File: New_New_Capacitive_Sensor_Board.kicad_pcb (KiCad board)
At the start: 4 copper layers, 23.9 x 21 mm, 17 parts, among them J1 Conn_01x04_Pin, J2 Conn_01x04_Pin, U1 FDC2212QDNTTQ1

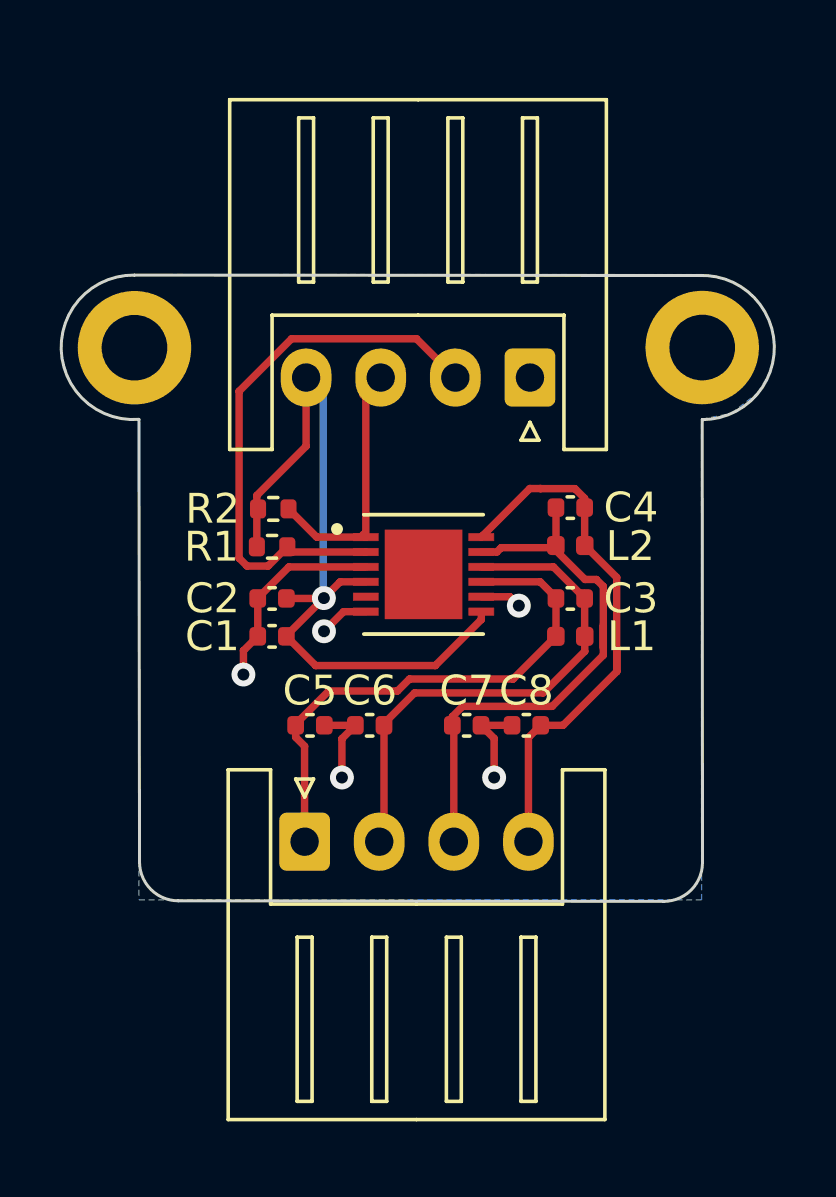
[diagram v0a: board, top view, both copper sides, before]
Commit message: needs gerber files
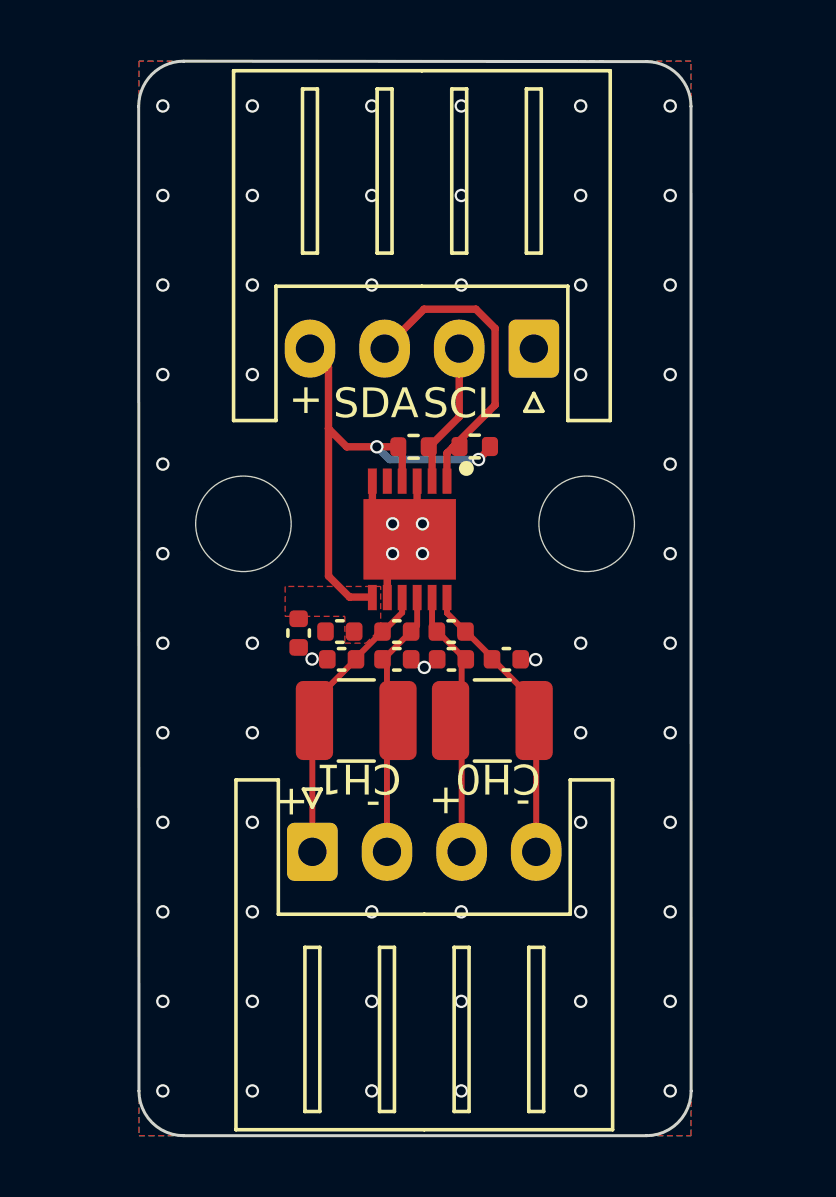
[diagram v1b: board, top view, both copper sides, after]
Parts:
- removed C1: 0.1u, Capacitor_SMD:C_0402_1005Metric
- removed C2: 1u, Capacitor_SMD:C_0402_1005Metric
- removed R1, R2: 1k, Resistor_SMD:R_0402_1005Metric
- removed REF** (x2): MountingHole_2.2mm_M2_DIN965_Pad, MountingHole:MountingHole_2.2mm_M2_DIN965_Pad
- removed U1: FDC2212QDNTTQ1, AD7150BRMZ:SON50P400X400X100-13N
- added C10: 1u, Capacitor_SMD:C_0402_1005Metric, F.Cu at (105.3, 63.2)
- added C9: 0.1u, Capacitor_SMD:C_0402_1005Metric, F.Cu at (106.7, 63.1)
- added G***: LOGO, iclr:nocap, B.Cu at (109.5, 62.4)
- added H1: MountingHole, MountingHole:MountingHole_3.2mm_M3_DIN965, F.Cu at (103.5, 59.5)
- added H2: MountingHole, MountingHole:MountingHole_3.2mm_M3_DIN965, F.Cu at (115.0, 59.5)
- added IC1: FDC2212QDNTTQ1, iclr:SON50P400X400X100-13N, F.Cu at (109.1, 60.0)
- added R3: 1k, Resistor_SMD:R_0402_1005Metric, F.Cu at (111.2, 56.9)
- added R4: 1k, Resistor_SMD:R_0402_1005Metric, F.Cu at (109.2, 56.9)
- L1, L2: footprint Inductor_SMD:L_0402_1005Metric -> Inductor_SMD:L_1210_3225Metric
- moved L1 7.71 mm to (107.3, 66.1)
- moved L2 6.42 mm to (111.8, 66.1)
- moved C3 5.92 mm to (108.6, 63.1)
- moved C4 5.76 mm to (110.5, 63.1)
- moved C5 2.45 mm to (106.8, 64.0), turned to 180 degrees
- moved C6 2.39 mm to (108.6, 64.0), turned to 180 degrees
- moved C8 2.31 mm to (112.3, 64.0), turned to 180 degrees
- moved C7 2.27 mm to (110.5, 64.0), turned to 180 degrees
- moved J1 0.98 mm to (113.2, 53.6)
- moved J2 0.43 mm to (105.8, 70.5)
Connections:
- net IN0A renamed IN0+
- net IN0B renamed IN0-
- net IN1A renamed IN1+
- net IN1B renamed IN1-
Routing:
- net SDA: track 18.8 -> 4.82 mm
- net IN1+: track 19.6 -> 9.06 mm
- net IN1-: track 19.1 -> 9.78 mm
- net GND: track 15.8 -> 6.78 mm, vias 5 -> 63
- net IN0-: track 17.6 -> 9.08 mm
- net IN0+: track 18.0 -> 9.78 mm
- net VDD: track 25.7 -> 17.6 mm, vias 1 -> 2
- net SCL: track 9.49 -> 10.3 mm
- added copper zone on F.Cu, net GND
- added copper zone on F.Cu, net VDD
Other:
- board size 23.9 x 21 mm -> 18.5 x 36 mm
- copper layers 4 -> 2
- board text added: "+"
- board text added: "-"
- board text added: "CH0"
- board text added: "CH1"
- board text added: "Designed by Toby Browne Electronics 2024"
- board text added: "SCL"
- board text added: "SDA"
